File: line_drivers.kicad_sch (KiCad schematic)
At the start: 20 parts, among them U3 SN74LVC8T245PWR, U4 SN74LVC8T245PWR, U5 MAX3232

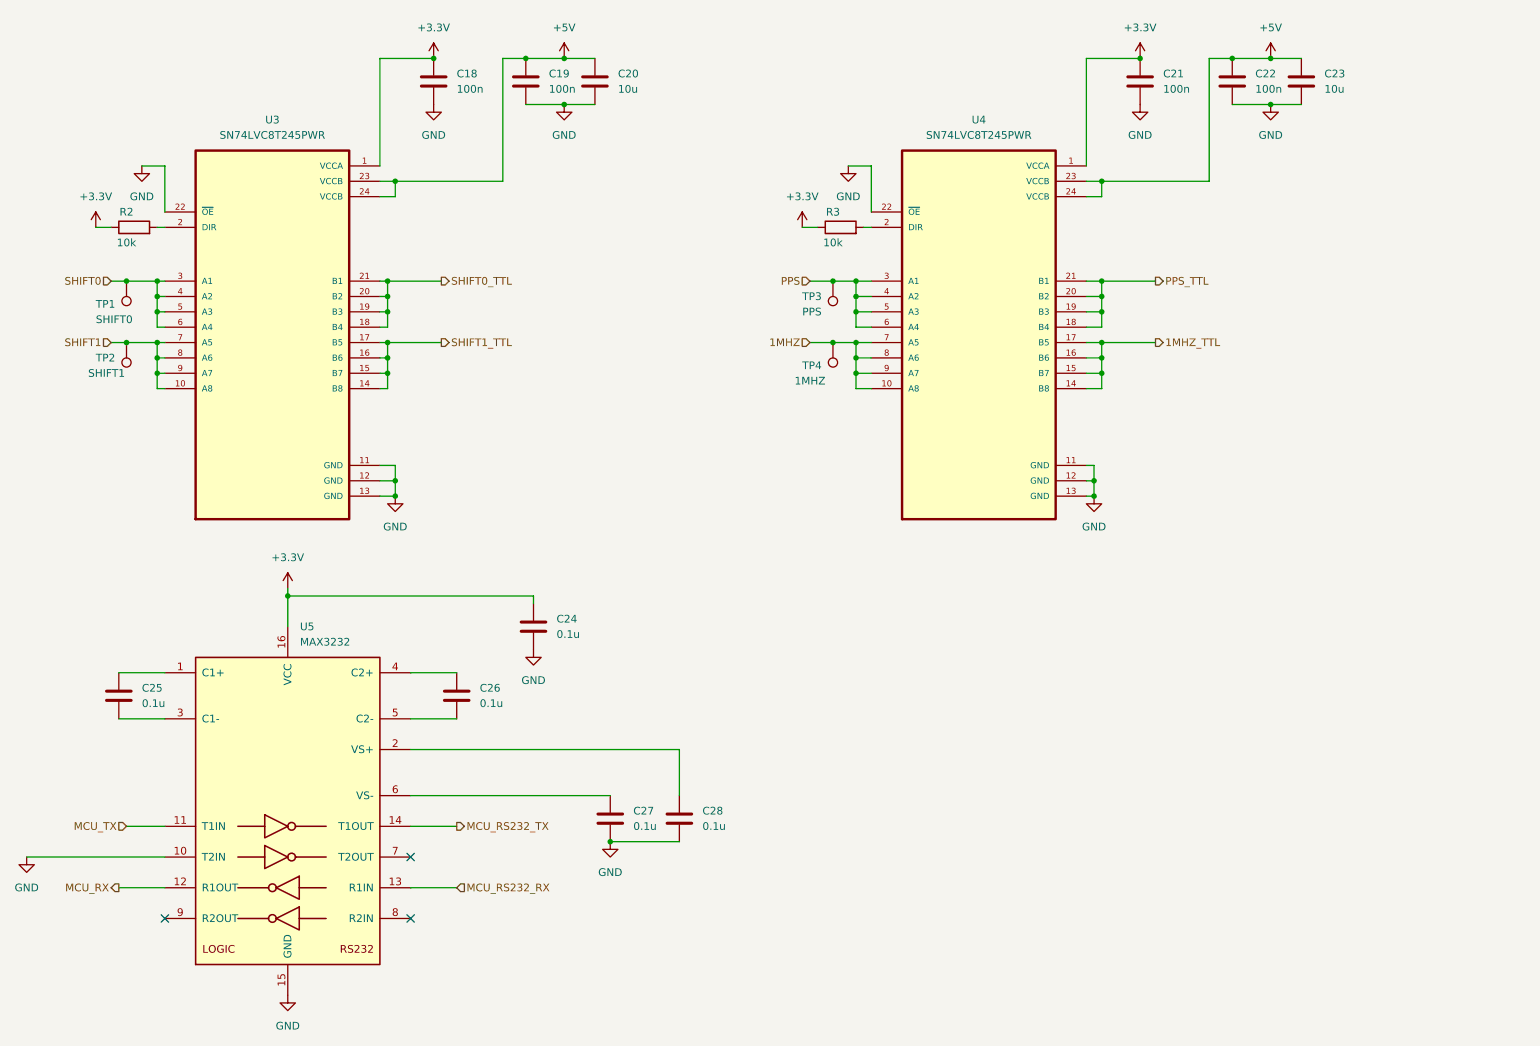
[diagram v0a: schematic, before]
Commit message: Rev3: Fix GPS receiver start problem and update to KiCad 7
- Pin TP2 of GPS receiver seems to be pulled down briefly at start time,
  this triggers the safe boot mode. A buffer was added to address this
  issue. Thanks Chris C. for the fix and thanks Paul H. for the
  investigation
- All files were adapted to KiCad 7 format and many symbols and footprints
  were replaced with newer ones.
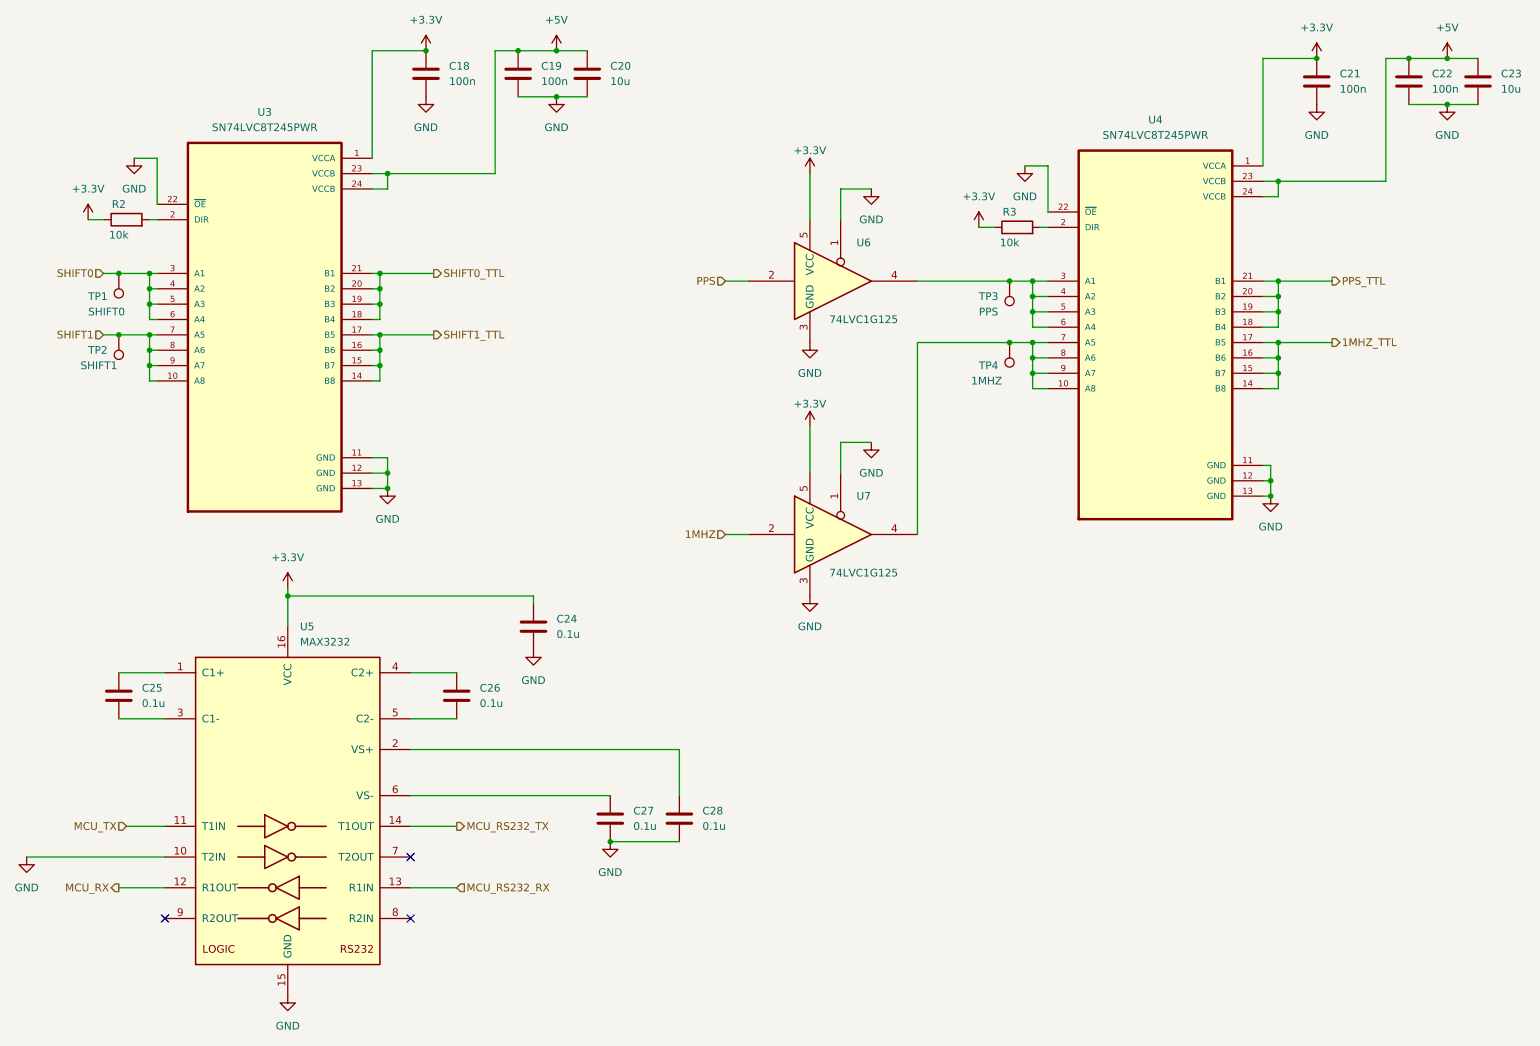
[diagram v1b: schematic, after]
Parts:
- added U6, U7: 74LVC1G125, Package_TO_SOT_SMD:SOT-23-5_HandSoldering, symbol 74xGxx:74LVC1G125
- U3, U4: footprint footprints:SOP65P640X120-24N -> Package_SO:TSSOP-24_4.4x7.8mm_P0.65mm
- U5: footprint footprints:SOIC127P600X175-16N -> Package_SO:SOIC-16_3.9x9.9mm_P1.27mm
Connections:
- net +3.3V: now also U6.5 (VCC), U7.5 (VCC)
- net 1MHZ: now also U7.2; no longer TP4.1, U4.10 (A8), U4.7 (A5), U4.8 (A6), U4.9 (A7)
- net GND: now also U6.1, U6.3 (GND), U7.1, U7.3 (GND)
- net PPS: now also U6.2; no longer TP3.1, U4.3 (A1), U4.4 (A2), U4.5 (A3), U4.6 (A4)
- new net: TP4.1, U4.10 (A8), U4.7 (A5), U4.8 (A6), U4.9 (A7), U7.4
- new net: TP3.1, U4.3 (A1), U4.4 (A2), U4.5 (A3), U4.6 (A4), U6.4
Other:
- moved on the sheet: C18, C19, C20, C21, C22, C23, R2, R3, TP1, TP2, TP3, TP4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
